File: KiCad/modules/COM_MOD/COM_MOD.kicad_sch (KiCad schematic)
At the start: 30 parts, among them J1 Conn_01x01_Pin, J11 Conn_01x01_Pin, J12 Conn_01x01_Pin, J13 Conn_01x01_Pin, J14 Conn_01x01_Pin, J15 Conn_01x01_Pin, J16 Conn_01x01_Pin, J17 Conn_01x01_Pin, J18 Conn_01x01_Pin, J19 Conn_01x01_Pin, J2 Conn_01x01_Pin, J20 Conn_01x01_Pin, J21 Conn_01x01_Pin, J22 Conn_01x01_Pin, J3 Conn_01x01_Pin, J5 Conn_01x01_Pin, J6 Conn_01x01_Pin, J7 Conn_01x01_Pin, J8 Conn_01x01_Pin, J9 Conn_01x01_Pin, SW1 NA, U1 HC32L110C6UA, U2 74HC688

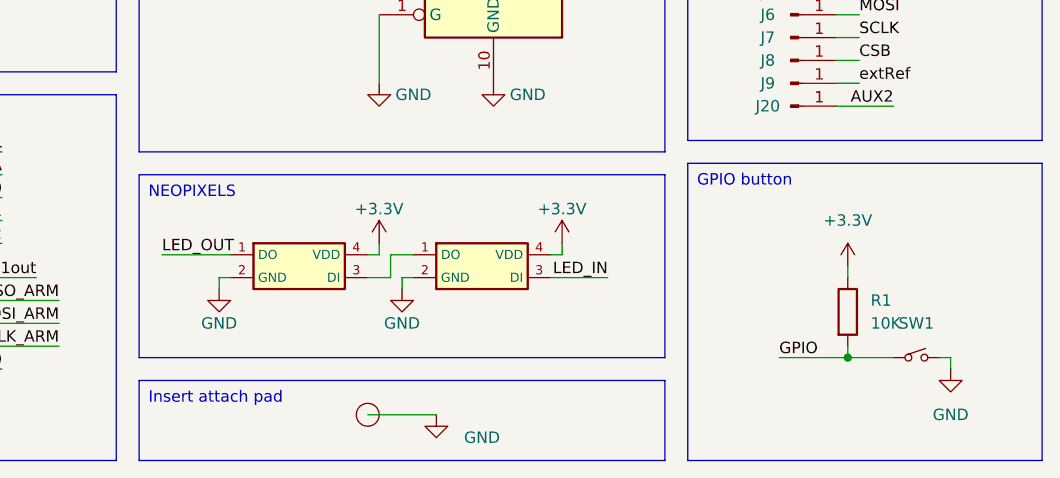
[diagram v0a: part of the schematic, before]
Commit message: updated
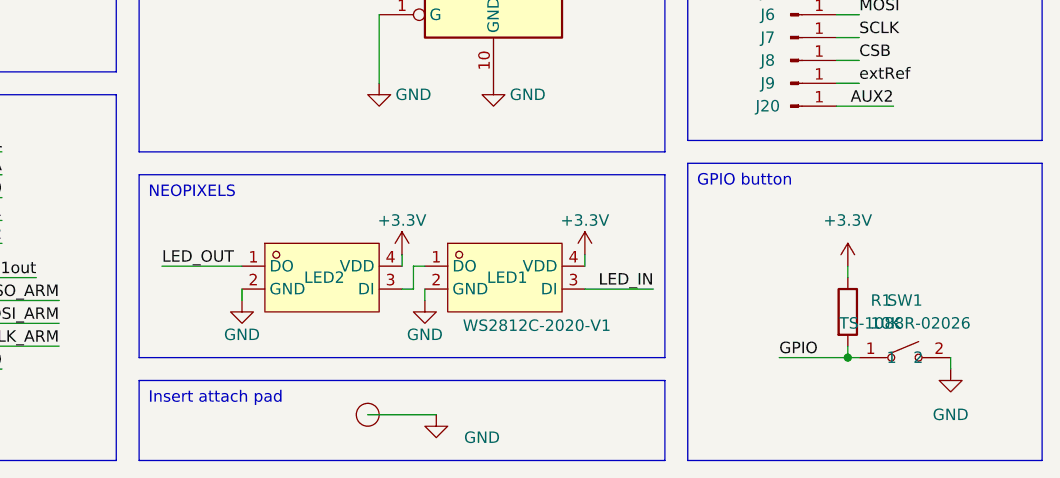
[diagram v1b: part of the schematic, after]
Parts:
- removed LED1, LED2: WS2812-2020, 00_Custom:WS2812-2020, symbol 00_custom:WS2812-2020
- removed SW1: NA, 00_Custom:SW-SMD_L3.9-W3.0-P4.45, symbol 00_custom:switch
- added LED1: WS2812C-2020-V1, 00_lcsc:LED-SMD_4P-L2.0-W2.0-TL_WS2812B-2020, symbol 00_lcsc:WS2812C-2020-V1
- added LED2: WS2812C, 00_lcsc:LED-SMD_4P-L2.0-W2.0-TL_WS2812B-2020, symbol 00_lcsc:WS2812C-2020-V1
- added SW1: TS-1088R-02026, 00_lcsc:SW-SMD_L3.9-W3.0-P4.45, symbol 00_lcsc:TS-1088R-02026
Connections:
- net +3.3V: now also LED1.4 (VDD), LED2.4 (VDD)
- net GND: now also LED1.2 (GND), LED2.2 (GND), SW1.2
- net GPIO: now also SW1.1
- net LED_IN: now also LED1.3 (DI)
- net LED_OUT: now also LED2.1 (DO)
- new net: LED1.1 (DO), LED2.3 (DI)
